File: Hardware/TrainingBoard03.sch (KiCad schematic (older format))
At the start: 3 parts

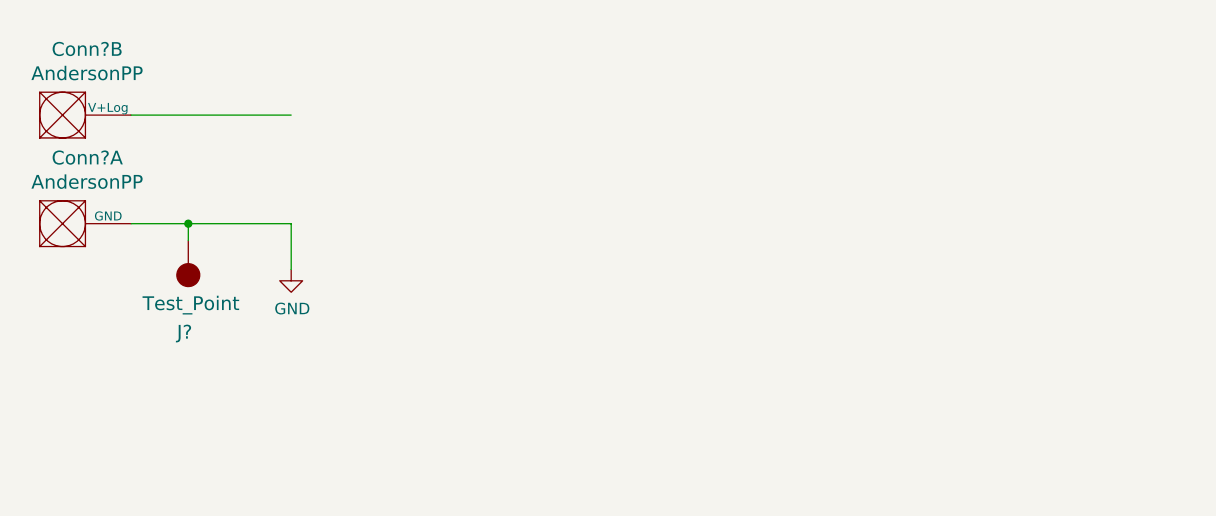
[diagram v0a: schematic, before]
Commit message: made board
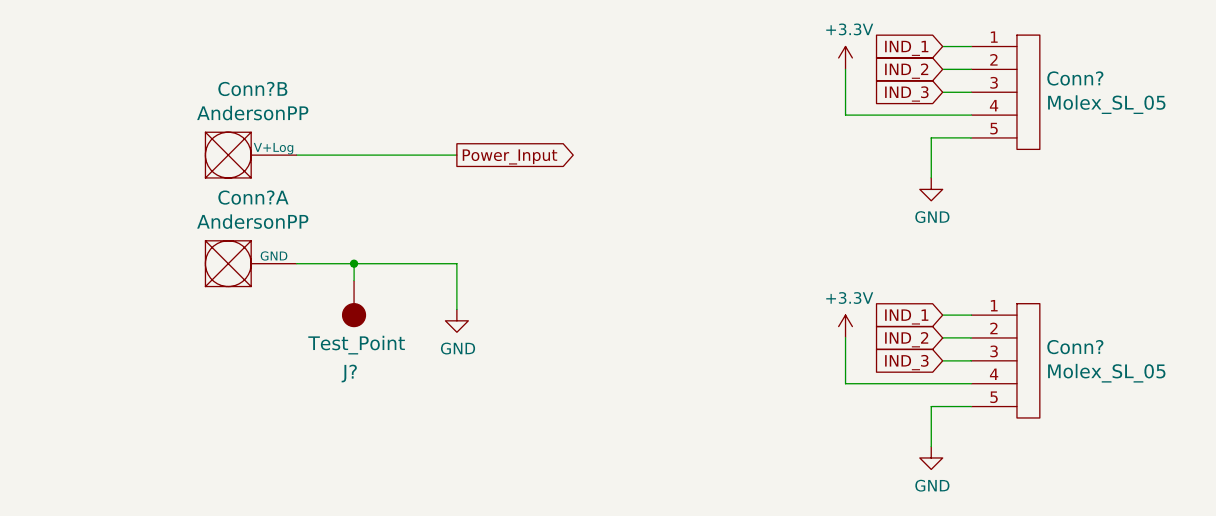
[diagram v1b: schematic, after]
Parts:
- added Conn? (x2): Molex_SL_05, symbol MRDT_Connectors:Molex_SL_05
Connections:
- net labels added: +3.3V, IND_1, IND_2, IND_3, Power_Input
- wire segments 5 -> 19
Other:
- moved on the sheet: Conn?A, Conn?B, J?
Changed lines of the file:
@@
 L MRDT_Connectors:AndersonPP Conn?
 U 1 1 5F579859
-P 2900 3650
-F 0 "Conn?" H 3108 4037 60  0000 C CNN
-F 1 "AndersonPP" H 3108 3931 60  0000 C CNN
-F 2 "" H 2750 3100 60  0001 C CNN
-F 3 "" H 2750 3100 60  0001 C CNN
-	1    2900 3650
+P 3625 3825
+AR Path="/5F525D93/5F579859" Ref="Conn?"  Part="1"
+AR Path="/5F5029F1/5F579859" Ref="Conn?"  Part="1"
+F 0 "Conn?" H 3833 4212 60  0000 C CNN
+F 1 "AndersonPP" H 3833 4106 60  0000 C CNN
+F 2 "" H 3475 3275 60  0001 C CNN
+F 3 "" H 3475 3275 60  0001 C CNN
+	1    3625 3825
 	1    0    0    -1
 $EndComp
@@
 L MRDT_Connectors:AndersonPP Conn?
 U 2 1 5F57985F
-P 2900 3175
-F 0 "Conn?" H 3108 3562 60  0000 C CNN
-F 1 "AndersonPP" H 3108 3456 60  0000 C CNN
-F 2 "" H 2750 2625 60  0001 C CNN
-F 3 "" H 2750 2625 60  0001 C CNN
-	2    2900 3175
+P 3625 3350
+AR Path="/5F525D93/5F57985F" Ref="Conn?"  Part="2"
+AR Path="/5F5029F1/5F57985F" Ref="Conn?"  Part="2"
+F 0 "Conn?" H 3833 3737 60  0000 C CNN
+F 1 "AndersonPP" H 3833 3631 60  0000 C CNN
+F 2 "" H 3475 2800 60  0001 C CNN
+F 3 "" H 3475 2800 60  0001 C CNN
+	2    3625 3350
 	1    0    0    -1
 $EndComp
 Wire Wire Line
-	3300 3550 3550 3550
+	4025 3725 4275 3725
 $Comp
 L MRDT_Connectors:Test_Point J?
 U 1 1 5F579866
-P 3550 3625
-F 0 "J?" H 3600 4025 60  0000 R CNN
-F 1 "Test_Point" H 3750 3900 60  0000 R CNN
-F 2 "" H 3550 3575 60  0001 C CNN
-F 3 "" H 3550 3575 60  0001 C CNN
-	1    3550 3625
+P 4275 3800
+AR Path="/5F525D93/5F579866" Ref="J?"  Part="1"
+AR Path="/5F5029F1/5F579866" Ref="J?"  Part="1"
+F 0 "J?" H 4325 4200 60  0000 R CNN
+F 1 "Test_Point" H 4475 4075 60  0000 R CNN
+F 2 "" H 4275 3750 60  0001 C CNN
+F 3 "" H 4275 3750 60  0001 C CNN
+	1    4275 3800
 	-1   0    0    1
 $EndComp
 Wire Wire Line
-	3550 3625 3550 3550
-Connection ~ 3550 3550
+	4275 3800 4275 3725
+Connection ~ 4275 3725
 Wire Wire Line
-	3550 3550 4000 3550
+	4275 3725 4725 3725
 Wire Wire Line
-	3300 3075 4000 3075
+	4025 3250 4725 3250
 Wire Wire Line
-	4000 3550 4000 3750
+	4725 3725 4725 3925
 $Comp
 L power:GND #PWR?
 U 1 1 5F5799A6
-P 4000 3750
-F 0 "#PWR?" H 4000 3500 50  0001 C CNN
-F 1 "GND" H 4005 3577 50  0000 C CNN
-F 2 "" H 4000 3750 50  0001 C CNN
-F 3 "" H 4000 3750 50  0001 C CNN
-	1    4000 3750
+P 4725 3925
+F 0 "#PWR?" H 4725 3675 50  0001 C CNN
+F 1 "GND" H 4730 3752 50  0000 C CNN
+F 2 "" H 4725 3925 50  0001 C CNN
+F 3 "" H 4725 3925 50  0001 C CNN
+	1    4725 3925
 	1    0    0    -1
 $EndComp
+Text GLabel 4725 3250 2    50   Output ~ 0
+Power_Input
+$Comp
+L MRDT_Connectors:Molex_SL_05 Conn?
+U 1 1 5F582D81
+P 7175 4400
+F 0 "Conn?" H 7303 4708 60  0000 L CNN
+F 1 "Molex_SL_05" H 7303 4602 60  0000 L CNN
+F 2 "" H 7175 4400 60  0001 C CNN
+F 3 "" H 7175 4400 60  0001 C CNN
+	1    7175 4400
+	1    0    0    -1
+$EndComp
+Wire Wire Line
+	6975 4350 6800 4350
+Wire Wire Line
+	6800 4350 6800 4525
+$Comp
+L power:GND #PWR?
+U 1 1 5F583AFF
+P 6800 4525
+F 0 "#PWR?" H 6800 4275 50  0001 C CNN
+F 1 "GND" H 6805 4352 50  0000 C CNN
+F 2 "" H 6800 4525 50  0001 C CNN
+F 3 "" H 6800 4525 50  0001 C CNN
+	1    6800 4525
+	1    0    0    -1
+$EndComp
+Wire Wire Line
+	6425 4250 6425 4050
+$Comp
+L power:+3.3V #PWR?
+U 1 1 5F583CFB
+P 6425 4050
+F 0 "#PWR?" H 6425 3900 50  0001 C CNN
+F 1 "+3.3V" H 6440 4223 50  0000 C CNN
+F 2 "" H 6425 4050 50  0001 C CNN
+F 3 "" H 6425 4050 50  0001 C CNN
+	1    6425 4050
+	1    0    0    -1
+$EndComp
+Wire Wire Line
+	6425 4250 6975 4250
+Text GLabel 6850 4150 0    50   Input ~ 0
+IND_3
+Text GLabel 6850 4050 0    50   Input ~ 0
+IND_2
+Text GLabel 6850 3950 0    50   Input ~ 0
+IND_1
+Wire Wire Line
+	6850 3950 6975 3950
+Wire Wire Line
+	6850 4050 6975 4050
+Wire Wire Line
+	6850 4150 6975 4150
+$Comp
+L MRDT_Connectors:Molex_SL_05 Conn?
+U 1 1 5F587554
+P 7175 3225
+F 0 "Conn?" H 7303 3533 60  0000 L CNN
+F 1 "Molex_SL_05" H 7303 3427 60  0000 L CNN
+F 2 "" H 7175 3225 60  0001 C CNN
+F 3 "" H 7175 3225 60  0001 C CNN
+	1    7175 3225
+	1    0    0    -1
+$EndComp
+Wire Wire Line
+	6975 3175 6800 3175
+Wire Wire Line
+	6800 3175 6800 3350
+$Comp
+L power:GND #PWR?
+U 1 1 5F58755C
+P 6800 3350
+F 0 "#PWR?" H 6800 3100 50  0001 C CNN
+F 1 "GND" H 6805 3177 50  0000 C CNN
+F 2 "" H 6800 3350 50  0001 C CNN
+F 3 "" H 6800 3350 50  0001 C CNN
+	1    6800 3350
+	1    0    0    -1
+$EndComp
+Wire Wire Line
+	6425 3075 6425 2875
+$Comp
+L power:+3.3V #PWR?
+U 1 1 5F587563
+P 6425 2875
+F 0 "#PWR?" H 6425 2725 50  0001 C CNN
+F 1 "+3.3V" H 6440 3048 50  0000 C CNN
+F 2 "" H 6425 2875 50  0001 C CNN
+F 3 "" H 6425 2875 50  0001 C CNN
+	1    6425 2875
+	1    0    0    -1
+$EndComp
+Wire Wire Line
+	6425 3075 6975 3075
+Text GLabel 6850 2975 0    50   Input ~ 0
+IND_3
+Text GLabel 6850 2875 0    50   Input ~ 0
+IND_2
+Text GLabel 6850 2775 0    50   Input ~ 0
+IND_1
+Wire Wire Line
+	6850 2775 6975 2775
+Wire Wire Line
+	6850 2875 6975 2875
+Wire Wire Line
+	6850 2975 6975 2975
 $EndSCHEMATC
